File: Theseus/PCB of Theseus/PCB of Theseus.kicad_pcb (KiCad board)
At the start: 2 copper layers, 125 x 70 mm, 94 parts, among them J1 Screw_Terminal_01x04, J10 Screw_Terminal_01x03, J2 Screw_Terminal_01x04, J3 Screw_Terminal_01x03, J4 Screw_Terminal_01x06, J5 Programmer, J6 Micro_SD_Card, J7 Screw_Terminal_01x02, J8 Screw_Terminal_01x06, J9 Screw_Terminal_01x03, Q1 NMOS, Q2 NMOS, U1 TPS564257DRL, U10 INA326, U2 MCP2562, U3 REF200, U4 INA326, U5 INA326, U6 STM32H750VBTx, U7 REF200, U8 MX25L25645G, U9 REF200

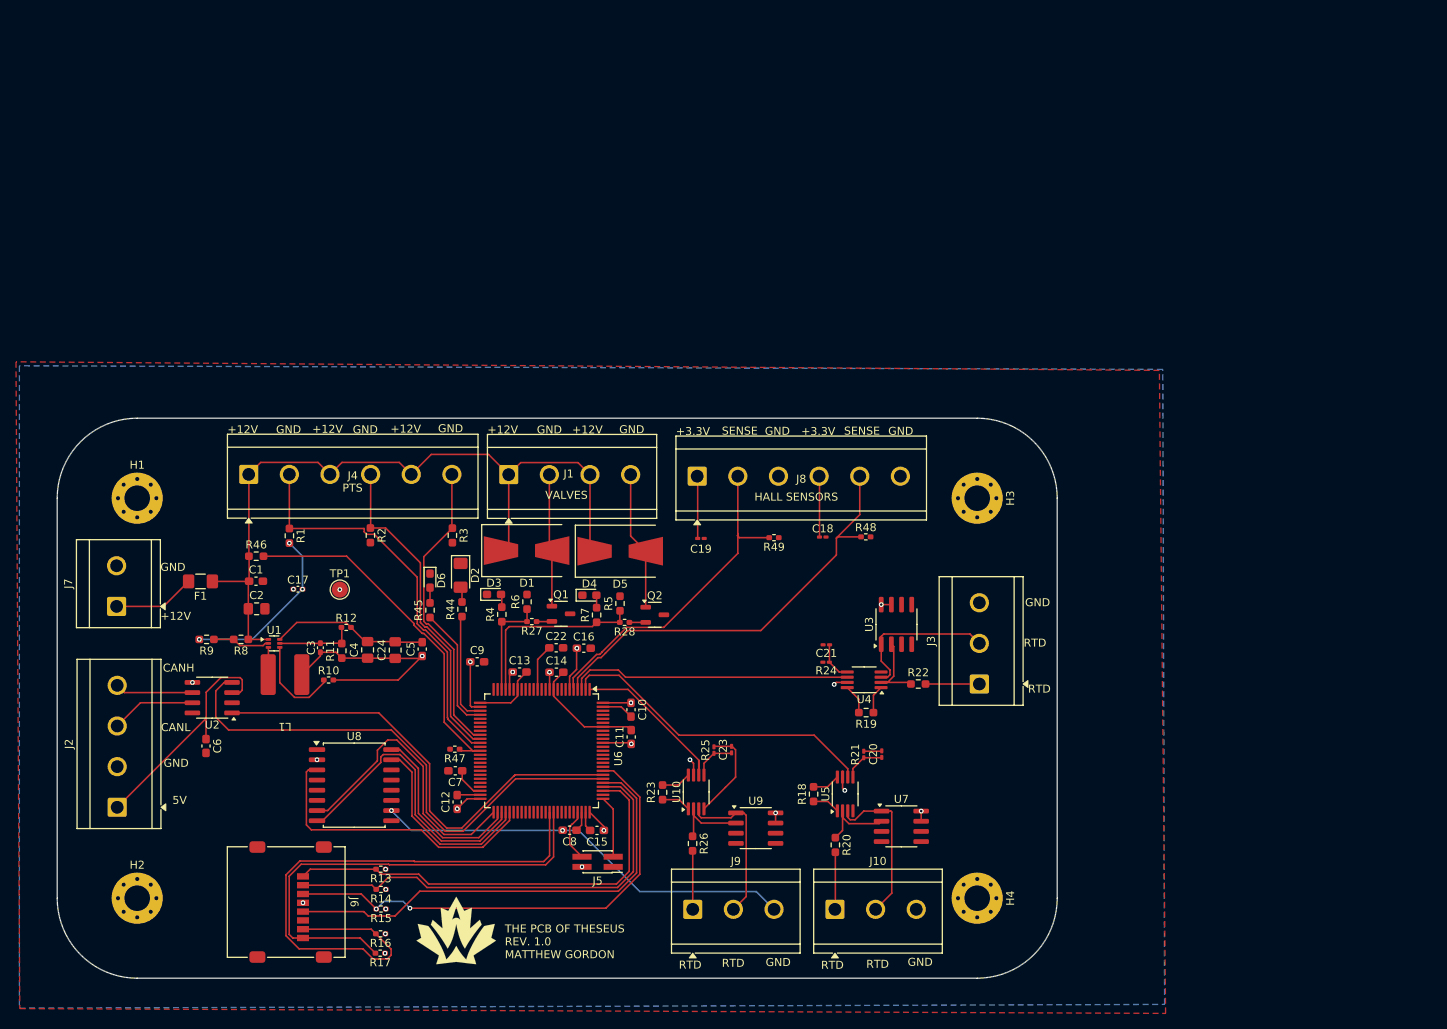
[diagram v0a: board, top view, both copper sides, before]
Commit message: Theseus_Dev_Rev2
It's still the same PCB
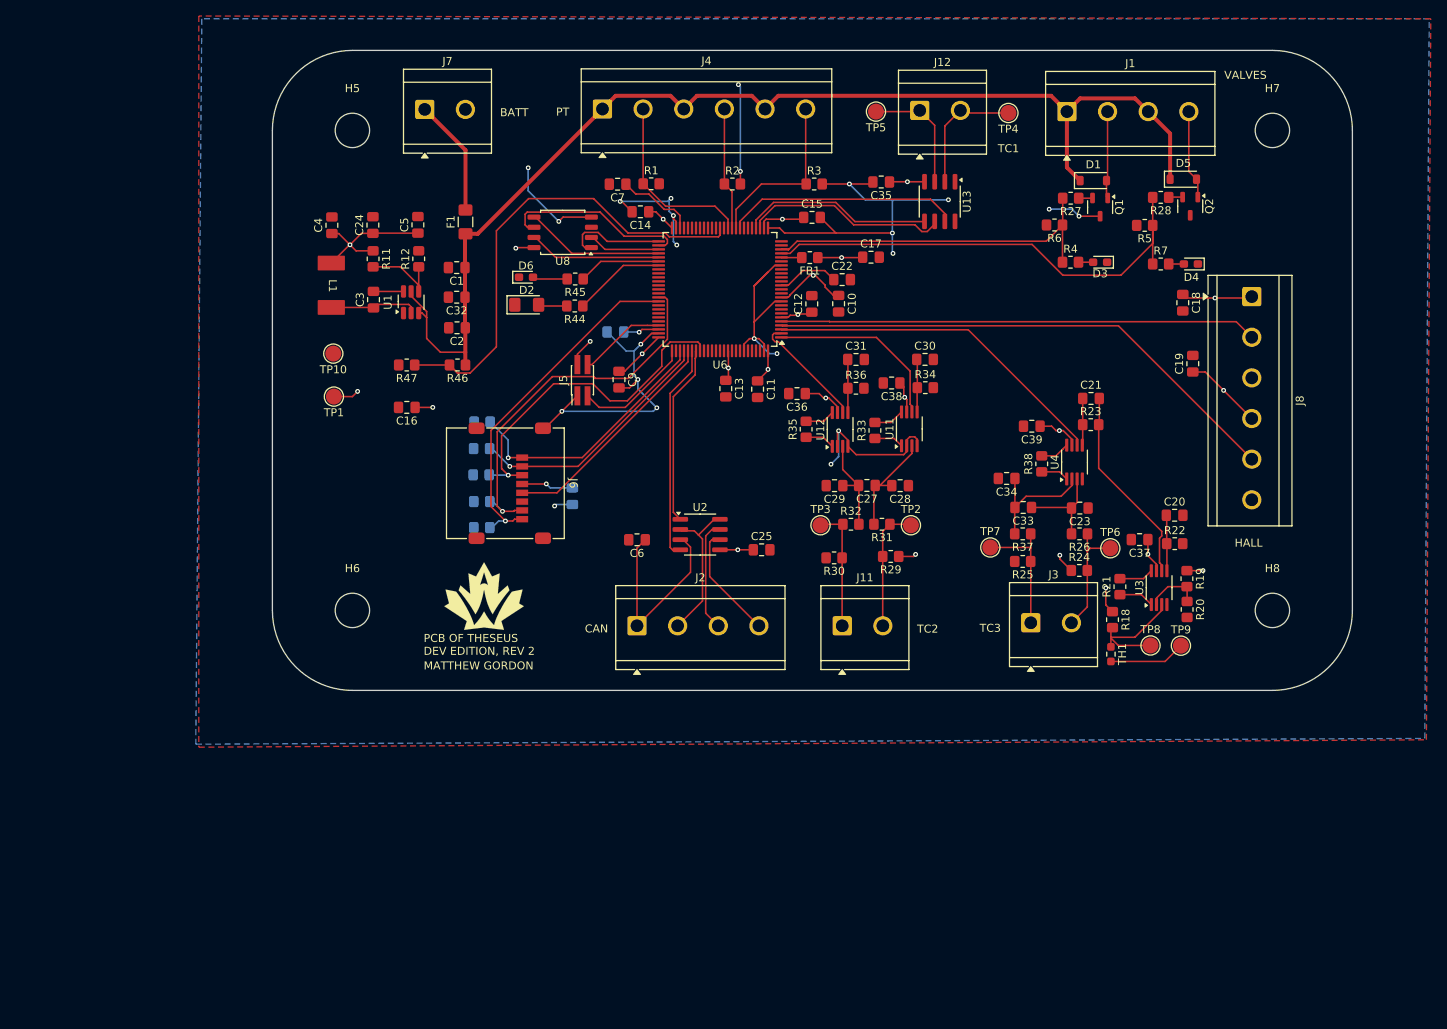
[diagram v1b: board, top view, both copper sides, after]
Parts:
- removed H1, H2, H3, H4: ~, MountingHole:MountingHole_3.2mm_M3_Pad_Via
- removed J10, J9: Screw_Terminal_01x03, TerminalBlock_CUI:TerminalBlock_CUI_TB007-508-03_1x03_P5.08mm_Horizontal
- removed R10: 10k, Resistor_SMD:R_0402_1005Metric_Pad0.72x0.64mm_HandSolder
- removed R48, R49: 3.4k, Resistor_SMD:R_0402_1005Metric_Pad0.72x0.64mm_HandSolder
- removed R8: 221k, Resistor_SMD:R_0603_1608Metric_Pad0.98x0.95mm_HandSolder
- removed R9: 30k, Resistor_SMD:R_0603_1608Metric_Pad0.98x0.95mm_HandSolder
- removed U10, U5: INA326, Package_SO:MSOP-8_3x3mm_P0.65mm
- removed U7, U9: REF200, Package_SO:SOIC-8_3.9x4.9mm_P1.27mm
- added C25: 10u, Capacitor_SMD:C_0805_2012Metric_Pad1.18x1.45mm_HandSolder, F.Cu at (144.5, 86.1)
- added C26: 10u, Capacitor_SMD:C_0805_2012Metric_Pad1.18x1.45mm_HandSolder, B.Cu at (120.8, 79.4)
- added C27: 0.047u, Capacitor_SMD:C_0805_2012Metric_Pad1.18x1.45mm_HandSolder, F.Cu at (157.7, 78.1)
- added C28: 0.47u, Capacitor_SMD:C_0805_2012Metric_Pad1.18x1.45mm_HandSolder, F.Cu at (161.8, 78.1)
- added C29: 0.47u, Capacitor_SMD:C_0805_2012Metric_Pad1.18x1.45mm_HandSolder, F.Cu at (153.6, 78.1)
- added C30: 2n, Capacitor_SMD:C_0805_2012Metric_Pad1.18x1.45mm_HandSolder, F.Cu at (164.9, 62.3)
- added C31: 2n, Capacitor_SMD:C_0805_2012Metric_Pad1.18x1.45mm_HandSolder, F.Cu at (156.3, 62.3)
- added C32: 10u, Capacitor_SMD:C_0805_2012Metric_Pad1.18x1.45mm_HandSolder, F.Cu at (106.4, 54.5)
- added C33: 0.047u, Capacitor_SMD:C_0805_2012Metric_Pad1.18x1.45mm_HandSolder, F.Cu at (177.2, 80.8)
- added C34: 0.47u, Capacitor_SMD:C_0805_2012Metric_Pad1.18x1.45mm_HandSolder, F.Cu at (175.1, 77.2)
- added C35: 0.1u, Capacitor_SMD:C_0805_2012Metric_Pad1.18x1.45mm_HandSolder, F.Cu at (159.4, 40.1)
- added C36: 0.1u, Capacitor_SMD:C_0805_2012Metric_Pad1.18x1.45mm_HandSolder, F.Cu at (148.9, 66.6)
- added C37: 0.1u, Capacitor_SMD:C_0805_2012Metric_Pad1.18x1.45mm_HandSolder, F.Cu at (191.8, 84.8)
- added C38: 0.1u, Capacitor_SMD:C_0805_2012Metric_Pad1.18x1.45mm_HandSolder, F.Cu at (160.8, 65.2)
- added C39: 0.1u, Capacitor_SMD:C_0805_2012Metric_Pad1.18x1.45mm_HandSolder, F.Cu at (178.3, 70.7)
- added FB1: FerriteBead, Resistor_SMD:R_0805_2012Metric_Pad1.20x1.40mm_HandSolder, F.Cu at (150.5, 49.6)
- added H5: MountingHole, MountingHole:MountingHole_4.3mm_M4, F.Cu at (93.3, 33.7)
- added H6: MountingHole, MountingHole:MountingHole_4.3mm_M4, F.Cu at (93.3, 93.7)
- added H7: MountingHole, MountingHole:MountingHole_4.3mm_M4, F.Cu at (208.3, 33.7)
- added H8: MountingHole, MountingHole:MountingHole_4.3mm_M4, F.Cu at (208.3, 93.7)
- added J11: TB002-500-02BE, TerminalBlock_CUI:TerminalBlock_CUI_TB007-508-02_1x02_P5.08mm_Horizontal, F.Cu at (154.6, 95.6)
- added J12: TB002-500-02BE, TerminalBlock_CUI:TerminalBlock_CUI_TB007-508-02_1x02_P5.08mm_Horizontal, F.Cu at (164.3, 31.2)
- added R29: 10M ±1%, Resistor_SMD:R_0805_2012Metric_Pad1.20x1.40mm_HandSolder, F.Cu at (160.6, 86.9)
- added R30: 1M ±0.1%, Resistor_SMD:R_0805_2012Metric_Pad1.20x1.40mm_HandSolder, F.Cu at (153.6, 87.1)
- added R31: 806R, Resistor_SMD:R_0805_2012Metric_Pad1.20x1.40mm_HandSolder, F.Cu at (159.5, 82.9)
- added R32: 806R, Resistor_SMD:R_0805_2012Metric_Pad1.20x1.40mm_HandSolder, F.Cu at (155.7, 82.9)
- added R33: 20k, Resistor_SMD:R_0805_2012Metric_Pad1.20x1.40mm_HandSolder, F.Cu at (158.7, 71.2)
- added R34: 80.6k, Resistor_SMD:R_0805_2012Metric_Pad1.20x1.40mm_HandSolder, F.Cu at (165.0, 65.8)
- added R35: 20k, Resistor_SMD:R_0805_2012Metric_Pad1.20x1.40mm_HandSolder, F.Cu at (150.1, 71.0)
- added R36: 80.6k, Resistor_SMD:R_0805_2012Metric_Pad1.20x1.40mm_HandSolder, F.Cu at (156.3, 65.9)
- added R37: 806R, Resistor_SMD:R_0805_2012Metric_Pad1.20x1.40mm_HandSolder, F.Cu at (177.1, 84.1)
- added R38: 8.06k, Resistor_SMD:R_0805_2012Metric_Pad1.20x1.40mm_HandSolder, F.Cu at (179.5, 75.4)
- added TH1: PTS060301B100RP100, Resistor_SMD:R_0603_1608Metric_Pad0.98x0.95mm_HandSolder, F.Cu at (188.2, 99.1)
- added TP10: TestPoint, TestPoint:TestPoint_Pad_D2.0mm, F.Cu at (91.0, 61.6)
- added TP2: TC2+, TestPoint:TestPoint_Pad_D2.0mm, F.Cu at (163.2, 83.0)
- added TP3: TC2-, TestPoint:TestPoint_Pad_D2.0mm, F.Cu at (151.9, 83.0)
- added TP4: TC1+, TestPoint:TestPoint_Pad_D2.0mm, F.Cu at (175.3, 31.5)
- added TP5: TC1-, TestPoint:TestPoint_Pad_D2.0mm, F.Cu at (158.8, 31.3)
- added TP6: TC3+, TestPoint:TestPoint_Pad_D2.0mm, F.Cu at (188.1, 85.9)
- added TP7: TC3-, TestPoint:TestPoint_Pad_D2.0mm, F.Cu at (173.1, 85.8)
- added TP8: RTD1, TestPoint:TestPoint_Pad_D2.0mm, F.Cu at (193.1, 98.1)
- added TP9: RTD2, TestPoint:TestPoint_Pad_D2.0mm, F.Cu at (196.9, 98.1)
- added U11: INA326, Package_SO:MSOP-8_3x3mm_P0.65mm, F.Cu at (163.0, 71.0)
- added U12: INA326, Package_SO:MSOP-8_3x3mm_P0.65mm, F.Cu at (154.3, 71.1)
- added U13: MAX6675, Package_SO:SOIC-8_3.9x4.9mm_P1.27mm, F.Cu at (166.8, 42.6)
- C1: value 100nF -> 10u; footprint Capacitor_SMD:C_0603_1608Metric_Pad1.08x0.95mm_HandSolder -> Capacitor_SMD:C_0805_2012Metric_Pad1.18x1.45mm_HandSolder
- C10, C11, C12, C13, C14, C15, C16, C22, C6, C7, C9: footprint Capacitor_SMD:C_0603_1608Metric_Pad1.08x0.95mm_HandSolder -> Capacitor_SMD:C_0805_2012Metric_Pad1.18x1.45mm_HandSolder
- C17: value 1u -> 1n; footprint Capacitor_SMD:C_0402_1005Metric_Pad0.74x0.62mm_HandSolder -> Capacitor_SMD:C_0805_2012Metric_Pad1.18x1.45mm_HandSolder
- C18, C19: value 0.1uF -> 0.1u; footprint Capacitor_SMD:C_0201_0603Metric_Pad0.64x0.40mm_HandSolder -> Capacitor_SMD:C_0805_2012Metric_Pad1.18x1.45mm_HandSolder
- C2: value 22uF -> 100n
- C20, C21: value 510pF -> 0.5n; footprint Capacitor_SMD:C_0201_0603Metric_Pad0.64x0.40mm_HandSolder -> Capacitor_SMD:C_0805_2012Metric_Pad1.18x1.45mm_HandSolder
- C23: value 510pF -> 0.47u; footprint Capacitor_SMD:C_0201_0603Metric_Pad0.64x0.40mm_HandSolder -> Capacitor_SMD:C_0805_2012Metric_Pad1.18x1.45mm_HandSolder
- C24, C4: value 22uF -> 22u
- C3: value 10pF -> 100n; footprint Capacitor_SMD:C_0402_1005Metric_Pad0.74x0.62mm_HandSolder -> Capacitor_SMD:C_0805_2012Metric_Pad1.18x1.45mm_HandSolder
- C5: value 100nF -> 22u; footprint Capacitor_SMD:C_0603_1608Metric_Pad1.08x0.95mm_HandSolder -> Capacitor_SMD:C_0805_2012Metric_Pad1.18x1.45mm_HandSolder
- C8: footprint Capacitor_SMD:C_0603_1608Metric_Pad1.08x0.95mm_HandSolder -> Capacitor_SMD:C_0805_2012Metric_Pad1.18x1.45mm_HandSolder; moved to B.Cu
- D1, D5: value D -> 1N4150-W-E3-18; footprint Diode_SMD:D_SMB-SMC_Universal_Handsoldering -> Diode_SMD:D_SOD-123
- F1: value TBD -> 3.5A 0685T3500-01
- J1, J2: value Screw_Terminal_01x04 -> TB001-500-04BE
- J3: value Screw_Terminal_01x03 -> TB002-500-02BE; footprint TerminalBlock_CUI:TerminalBlock_CUI_TB007-508-03_1x03_P5.08mm_Horizontal -> TerminalBlock_CUI:TerminalBlock_CUI_TB007-508-02_1x02_P5.08mm_Horizontal
- J4, J8: value Screw_Terminal_01x06 -> TB003-500-P06BE
- J5: value Programmer -> Programmer GRPB022VWQS-RC
- J6: value Micro_SD_Card -> Micro SD Holder 0472192001
- J7: value Screw_Terminal_01x02 -> TB002-500-02BE
- L1: value 3.3uH -> 2.2u; footprint Fydp_footprints:VLS6045EX-3R3N -> Fydp_footprints:SPM6530T-2R2M
- Q1, Q2: value NMOS -> NX3020NAK,215
- R1, R2, R3: value 150R -> 150R ±0.1%; footprint Resistor_SMD:R_0603_1608Metric_Pad0.98x0.95mm_HandSolder -> Resistor_SMD:R_0805_2012Metric_Pad1.20x1.40mm_HandSolder
- R11: value 45.3k -> 33.2k; footprint Resistor_SMD:R_0603_1608Metric_Pad0.98x0.95mm_HandSolder -> Resistor_SMD:R_0805_2012Metric_Pad1.20x1.40mm_HandSolder
- R12: value 10k -> 10.2k; footprint Resistor_SMD:R_0402_1005Metric_Pad0.72x0.64mm_HandSolder -> Resistor_SMD:R_0805_2012Metric_Pad1.20x1.40mm_HandSolder
- R13, R14, R15, R16, R17: footprint Resistor_SMD:R_0402_1005Metric_Pad0.72x0.64mm_HandSolder -> Resistor_SMD:R_0805_2012Metric_Pad1.20x1.40mm_HandSolder; moved to B.Cu
- R18, R19: value 2k -> 32.4k ±0.1%; footprint Resistor_SMD:R_0603_1608Metric_Pad0.98x0.95mm_HandSolder -> Resistor_SMD:R_0805_2012Metric_Pad1.20x1.40mm_HandSolder
- R20: value 76.8R -> 100R ±0.1%; footprint Resistor_SMD:R_0603_1608Metric_Pad0.98x0.95mm_HandSolder -> Resistor_SMD:R_0805_2012Metric_Pad1.20x1.40mm_HandSolder
- R21: value 324k -> 8.06k; footprint Resistor_SMD:R_0201_0603Metric_Pad0.64x0.40mm_HandSolder -> Resistor_SMD:R_0805_2012Metric_Pad1.20x1.40mm_HandSolder
- R22: value 76.8R -> 200k; footprint Resistor_SMD:R_0603_1608Metric_Pad0.98x0.95mm_HandSolder -> Resistor_SMD:R_0805_2012Metric_Pad1.20x1.40mm_HandSolder
- R23: value 2k -> 200k; footprint Resistor_SMD:R_0603_1608Metric_Pad0.98x0.95mm_HandSolder -> Resistor_SMD:R_0805_2012Metric_Pad1.20x1.40mm_HandSolder
- R24, R25: value 324k -> 1M ±0.1%; footprint Resistor_SMD:R_0201_0603Metric_Pad0.64x0.40mm_HandSolder -> Resistor_SMD:R_0805_2012Metric_Pad1.20x1.40mm_HandSolder
- R26: value 76.8R -> 806R; footprint Resistor_SMD:R_0603_1608Metric_Pad0.98x0.95mm_HandSolder -> Resistor_SMD:R_0805_2012Metric_Pad1.20x1.40mm_HandSolder
- R27, R28: footprint Resistor_SMD:R_0402_1005Metric_Pad0.72x0.64mm_HandSolder -> Resistor_SMD:R_0805_2012Metric_Pad1.20x1.40mm_HandSolder
- R4, R44, R45, R5, R6, R7: footprint Resistor_SMD:R_0603_1608Metric_Pad0.98x0.95mm_HandSolder -> Resistor_SMD:R_0805_2012Metric_Pad1.20x1.40mm_HandSolder
- R46: value 30K -> 3M ±1%; footprint Resistor_SMD:R_0603_1608Metric_Pad0.98x0.95mm_HandSolder -> Resistor_SMD:R_0805_2012Metric_Pad1.20x1.40mm_HandSolder
- R47: value 10K -> 1M ±0.1%; footprint Resistor_SMD:R_0402_1005Metric_Pad0.72x0.64mm_HandSolder -> Resistor_SMD:R_0805_2012Metric_Pad1.20x1.40mm_HandSolder
- U1: value TPS564257DRL -> TPS565201DDC; footprint Package_TO_SOT_SMD:SOT-563 -> Package_TO_SOT_SMD:SOT-23-6_Handsoldering
- U3: value REF200 -> INA326; footprint Package_SO:SOIC-8_3.9x4.9mm_P1.27mm -> Package_SO:MSOP-8_3x3mm_P0.65mm
- U8: footprint Package_SO:SOIC-16W_7.5x10.3mm_P1.27mm -> Package_SO:SOIC-8_5.3x5.3mm_P1.27mm
- moved D3 86.4 mm to (186.8, 50.1), turned to 180 degrees
- moved D4 85.8 mm to (198.2, 50.4), turned to 180 degrees
- moved R27 85.7 mm to (183.1, 42.1)
- moved R28 85.5 mm to (194.4, 42.0)
- moved D1 84.6 mm to (186.0, 40.0)
- moved Q1 84.4 mm to (186.8, 43.3), turned to -90 degrees
- moved D5 84.4 mm to (197.2, 39.8)
- moved Q2 84.2 mm to (198.1, 43.1), turned to -90 degrees
- moved R4 83.6 mm to (183.1, 50.1), turned to 0 degrees
- moved J1 83.2 mm to (182.7, 31.3)
- moved R7 83.1 mm to (194.4, 50.4), turned to 0 degrees
- moved C17 82.8 mm to (158.2, 49.5)
- moved C15 81.2 mm to (150.8, 44.5), turned to 0 degrees
- moved R6 81.0 mm to (181.1, 45.5), turned to 180 degrees
- moved R5 80.8 mm to (192.4, 45.5), turned to 180 degrees
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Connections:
- net /MCU/RTD_1 renamed /MCU/TC3
- C20 pad 1: Net-(U5-R2) -> Net-(U3-R2)
- C21 pad 2: GND -> Net-(C21-Pad2)
- C23 pad 1: Net-(U10-R2) -> GND
- C23 pad 2: GND -> Net-(U4-+)
- C3 pad 1: +3.3V -> Net-(U1-SW)
- C3 pad 2: Net-(U1-FB) -> Net-(U1-VBST)
- R11 pad 2: Net-(U1-FB) -> Net-(U1-VFB)
- R12 pad 1: Net-(U1-FB) -> Net-(U1-VFB)
- R18 pad 1: Net-(R18-Pad1) -> +3.3V
- R18 pad 2: Net-(R18-Pad2) -> /Temperature Sensors/RTD+
- R19 pad 1: Net-(R19-Pad1) -> +3.3V
- R19 pad 2: Net-(R19-Pad2) -> Net-(U3--)
- R20 pad 1: Net-(U5--) -> Net-(U3--)
- R20 pad 2: Net-(J10-Pin_1) -> GND
- R21 pad 1: Net-(U5-R2) -> Net-(R21-Pad1)
- R21 pad 2: GND -> Net-(R21-Pad2)
- R22 pad 1: Net-(U3-I2_LOW) -> Net-(U3-R2)
- R22 pad 2: Net-(J3-Pin_1) -> GND
- R23 pad 1: Net-(R23-Pad1) -> Net-(U4-R2)
- R23 pad 2: Net-(R23-Pad2) -> Net-(C21-Pad2)
- R24 pad 1: Net-(U4-R2) -> +3.3V
- R24 pad 2: GND -> Net-(J3-Pin_2)
- R25 pad 1: Net-(U10-R2) -> Net-(J3-Pin_1)
- R26 pad 1: Net-(U10--) -> Net-(J3-Pin_2)
- R26 pad 2: Net-(J9-Pin_1) -> Net-(U4-+)
- U1 pad 1: +BATT -> GND
- U1 pad 2: Net-(U1-EN) -> Net-(U1-SW)
- U1 pad 3: Net-(U1-SW) -> +BATT
- U1 pad 4: Net-(U1-PG) -> Net-(U1-VFB)
- U1 pad 5: Net-(U1-FB) -> +BATT
- U1 pad 6: GND -> Net-(U1-VBST)
- U3 pad 1: Net-(J3-Pin_2) -> Net-(R21-Pad1)
- U3 pad 2: Net-(U3-I2_LOW) -> Net-(U3--)
- U3 pad 3: unconnected-(U3-MIRROR_COMMON-Pad3) -> /Temperature Sensors/RTD+
- U3 pad 4: unconnected-(U3-MIRROR_OUTPUT-Pad4) -> GND
- U3 pad 5: unconnected-(U3-MIRROR_INPUT-Pad5) -> Net-(U3-R2)
- U3 pad 6: unconnected-(U3-SUBSTRATE-Pad6) -> Net-(C21-Pad2)
- U3 pad 8: +3.3V -> Net-(R21-Pad2)
- U4 pad 1: Net-(R19-Pad1) -> Net-(R38-Pad1)
- U4 pad 2: Net-(U3-I2_LOW) -> Net-(U4--)
- U4 pad 3: Net-(J3-Pin_2) -> Net-(U4-+)
- U4 pad 8: Net-(R19-Pad2) -> Net-(R38-Pad2)
- U6 pad 1: /MCU/RTD_3 -> /MCU/TC2+
- U6 pad 2: /MCU/RTD_2 -> /MCU/TC2-
- U6 pad 21: +3.3V -> Net-(U6-VDDA)
- U6 pad 28: /MCU/LED_BLUE -> /MCU/TC1_NSS
- U6 pad 29: /MCU/LED_RED -> /MCU/TC1_SCK
- U6 pad 33: unconnected-(U6-PC5-Pad33) -> /MCU/TC1_SI
- U6 pad 56: unconnected-(U6-PD9-Pad56) -> /MCU/LED_RED
- U6 pad 57: unconnected-(U6-PD10-Pad57) -> /MCU/LED_BLUE
- U8 pad 1: unconnected-(U8-NC/SOIC3-Pad1) -> /MCU/SPI_NSS
- U8 pad 2: +3.3V -> /MCU/SPI_MISO
- U8 pad 3: /MCU/MEM_~{RESET} -> unconnected-(U8-WP#/SIO2-Pad3)
- U8 pad 4: unconnected-(U8-NC-Pad4) -> GND
- U8 pad 5: unconnected-(U8-NC-Pad5) -> /MCU/SPI_MOSI
- U8 pad 6: unconnected-(U8-NC-Pad6) -> /MCU/SPI_SCK
- U8 pad 7: /MCU/SPI_NSS -> /MCU/MEM_~{RESET}
- U8 pad 8: /MCU/SPI_MISO -> +3.3V
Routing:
- net GND: track 141.8 -> 208.8 mm, vias 5 -> 23
- net +3.3V: track 85.2 -> 137.4 mm
- net +BATT: track 96.0 -> 146.3 mm
- net /MCU/RTD_2: track 40.1 -> 0.00 mm
- net /CAN_Rx: track 66.2 -> 27.1 mm
- net /MCU/VALVE_2: track 23.6 -> 60.7 mm
- net /CAN_Tx: track 58.6 -> 22.6 mm
- net /MCU/VALVE_1: track 13.2 -> 44.6 mm
- net /MCU/SD_CLK: track 58.5 -> 28.9 mm
- net /MCU/TC1_SI: track 0.00 -> 29.3 mm
- net /MCU/SD_D0: track 75.2 -> 47.3 mm, vias 0 -> 1
- net /MCU/SPI_MISO: track 36.7 -> 9.02 mm
- net /MCU/PT_1: track 50.3 -> 22.9 mm
- net /MCU/TC1_NSS: track 0.00 -> 25.6 mm
- net /MCU/PT_2: track 40.5 -> 15.3 mm
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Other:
- board size 125 x 70 mm -> 135 x 80 mm
- board text added: "BATT"
- board text added: "CAN"
- board text added: "HALL"
- board text added: "MATTHEW GORDON"
- board text added: "PCB OF THESEUS DEV EDITION, REV 2"
- board text added: "PT"
- board text added: "TC1"
- board text added: "TC2"
- board text added: "TC3"
- board text removed: "+12V"
- board text removed: "+3.3V"
- board text removed: "5V"
- board text removed: "CANH"
- board text removed: "CANL"
- board text removed: "GND"
- board text removed: "HALL SENSORS"
- board text removed: "IF YOU'RE READING THIS, YOU'RE HOLDING THE PCB UPSIDE DOWN"
- board text removed: "PTS"
- board text removed: "RTD"
- board text removed: "SENSE"
- board text removed: "THE PCB OF THESEUS REV. 1.0 MATTHEW GORDON"
